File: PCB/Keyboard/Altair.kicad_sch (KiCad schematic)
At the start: 6 parts, among them J1 Conn_01x02_Socket, SW97 SW_Nidec_CAS-120A1, SW98 RotaryEncoder_Switch, SW99 SW_Push, U1 SuperMini nRF52840

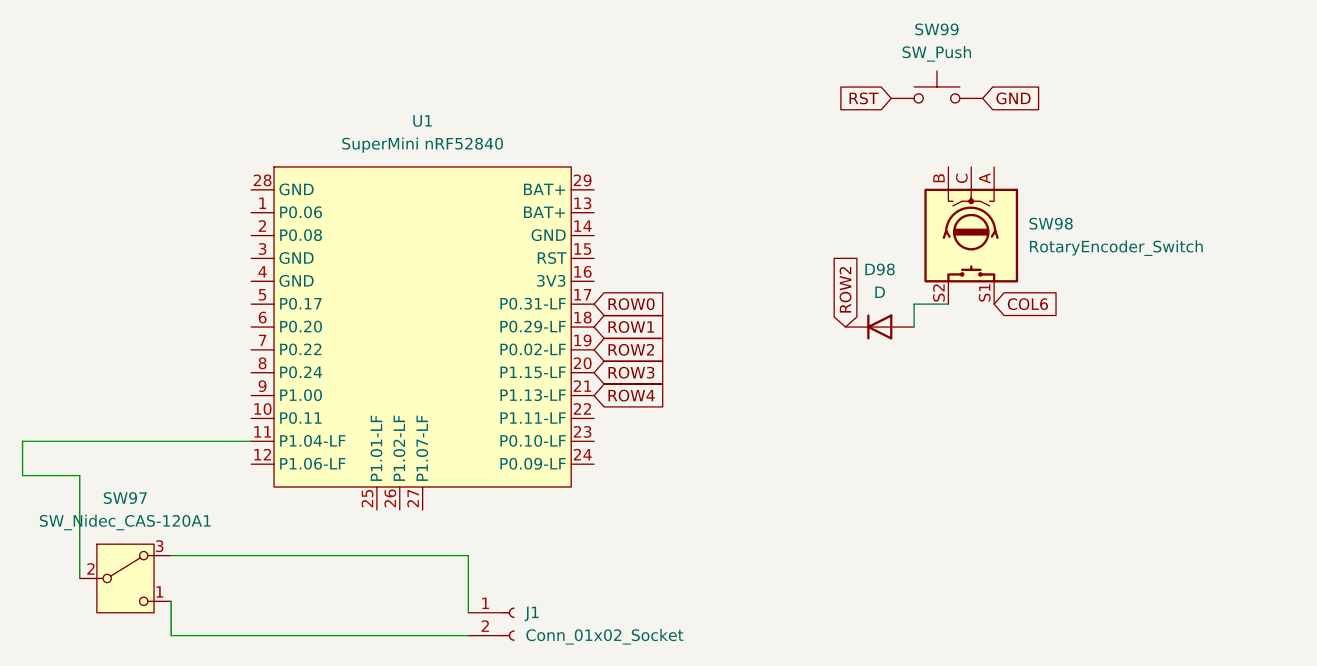
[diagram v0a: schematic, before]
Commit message: inprocess
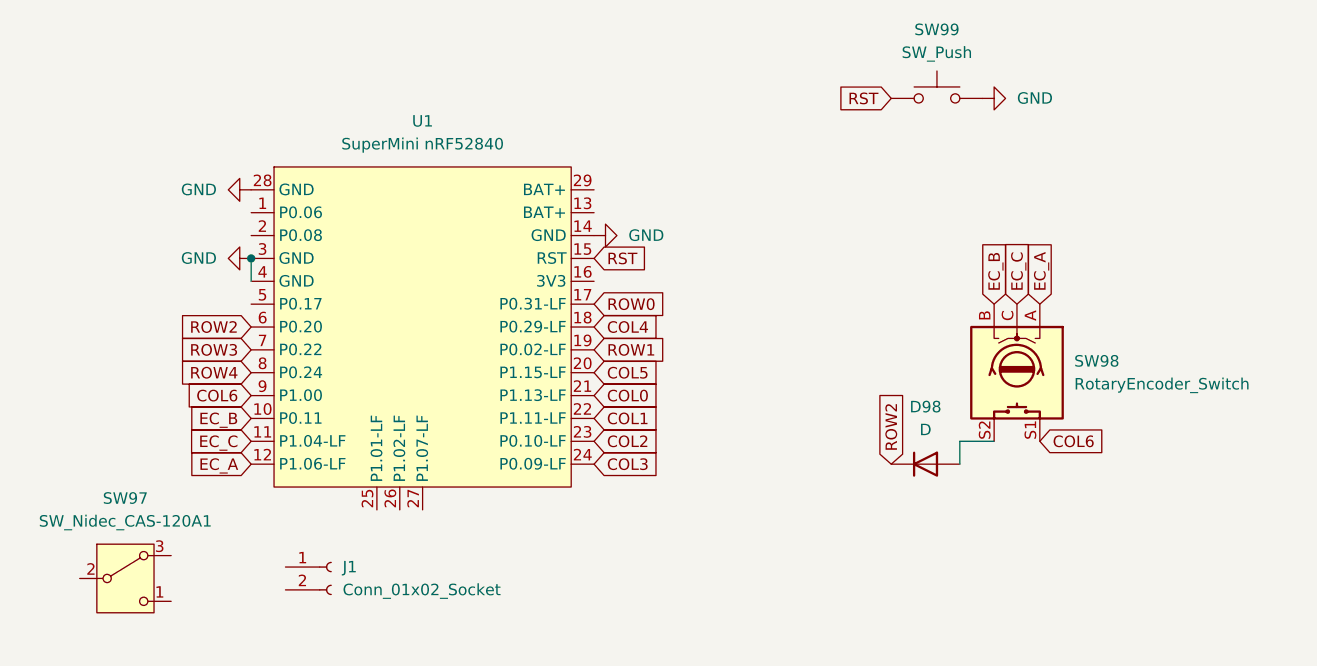
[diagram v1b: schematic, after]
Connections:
- net COL6: now also U1.9 (P1.00)
- net GND: now also U1.14 (GND), U1.28 (GND), U1.3 (GND), U1.4 (GND)
- net ROW1: now also U1.19 (P0.02-LF); no longer U1.18 (P0.29-LF)
- net ROW2: now also U1.6 (P0.20); no longer U1.19 (P0.02-LF)
- net ROW3: now also U1.7 (P0.22); no longer U1.20 (P1.15-LF)
- net ROW4: now also U1.8 (P0.24); no longer U1.21 (P1.13-LF)
- net RST: now also U1.15 (RST)
- net EC_B: now reaches U1.10 (P0.11)
- net EC_B: now also SW98.B
- net at SW97.2 (B): no longer U1.11 (P1.04-LF)
- net EC_A: now reaches U1.12 (P1.06-LF)
- net EC_A: now also SW98.A
- net COL1: now reaches U1.22 (P1.11-LF)
- net COL2: now reaches U1.23 (P0.10-LF)
- net COL3: now reaches U1.24 (P0.09-LF)
- net at SW97.1 (C): no longer J1.2 (Pin_2)
- net at SW97.3 (A): no longer J1.1 (Pin_1)
- net EC_C: now reaches SW98.C
- net EC_C: now also U1.11 (P1.04-LF)
- new net COL0: U1.21 (P1.13-LF)
- new net COL4: U1.18 (P0.29-LF)
- new net COL5: U1.20 (P1.15-LF)
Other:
- moved on the sheet: D98, J1, SW98
